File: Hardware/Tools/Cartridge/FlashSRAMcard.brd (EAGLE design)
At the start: 47.9 x 47.9 mm, 18 parts, among them IC1 AS29CF160B-55TIN, IC2 74LS595D, IC3 74LS244DW, IC5 74AHC1G04DBV, IC6 74AHC1G32DBV, IC7 74AHC1G32DBV

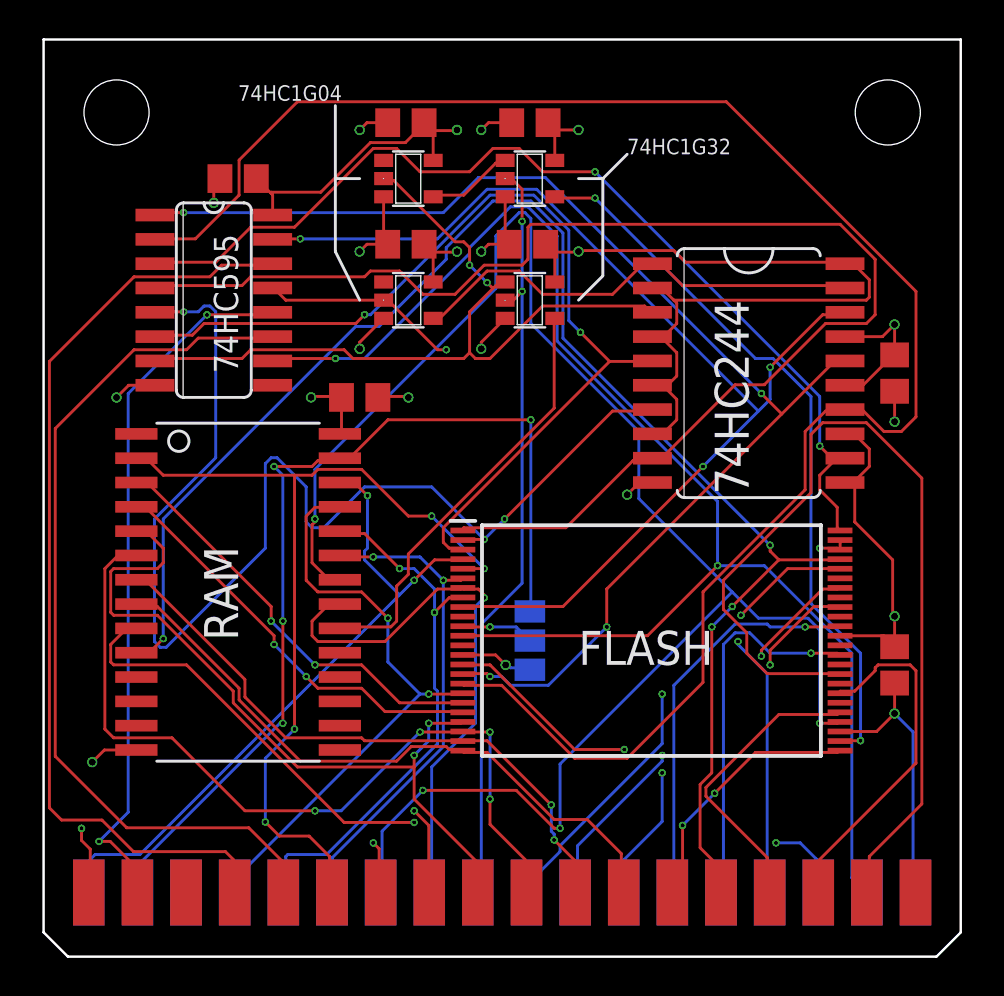
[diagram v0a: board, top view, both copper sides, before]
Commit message: more sram cart changes
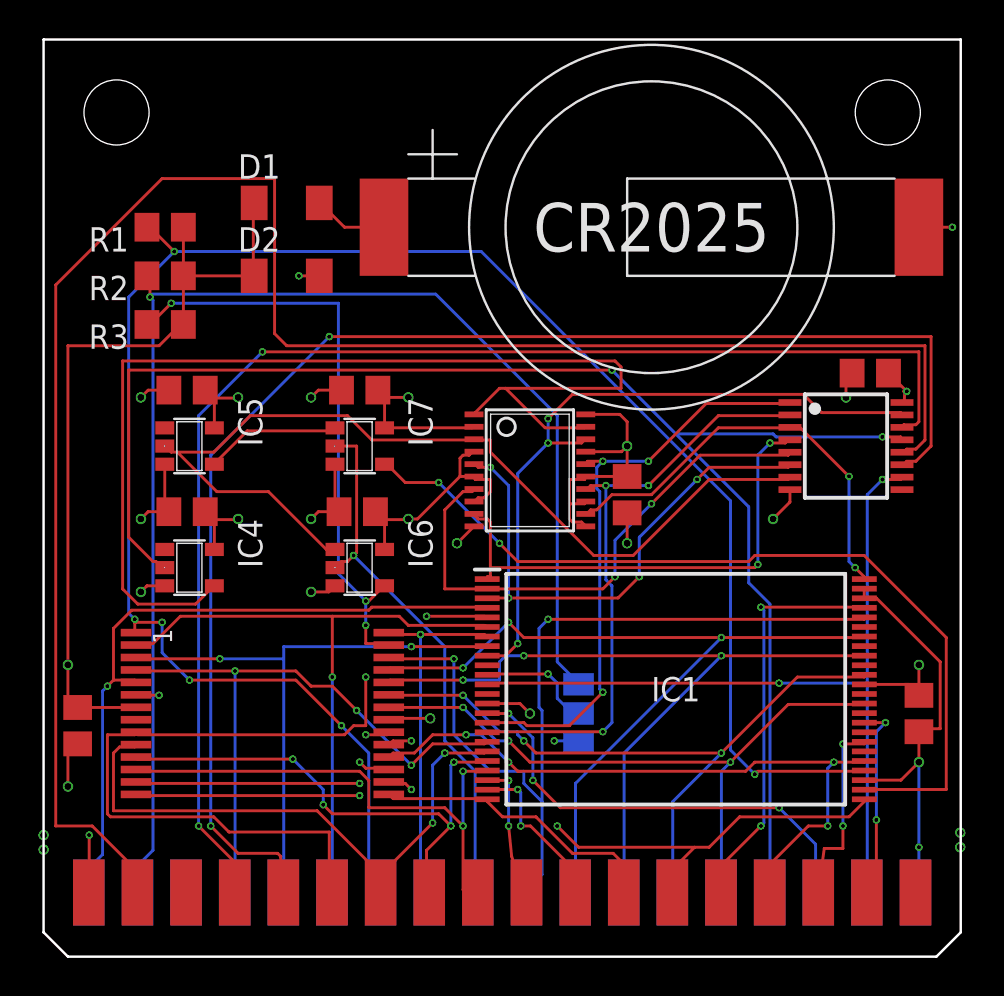
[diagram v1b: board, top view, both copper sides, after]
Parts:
- removed VCC: 74AHC1G04DBV, 74xx-little-us:SOT23-5
- added D1, D2: (no value), semicon-smd-ipc:MELF-MLL34
- added IC4: 74AHC1G04DBV, 74xx-little-us:SOT23-5
- added R1, R2, R3: (no value), rcl:R0805
- added U$3: BATTERY2025-SMD, 0_gametankparts:CR2025-SMD
- IC2: value 74LS595D -> 74HC595; device 74xx-us:SO16 -> 0_gametankparts:TSSOP16
- IC3: value 74LS244DW -> 74HC244; device 74xx-us:SO20W -> 0_gametankparts:TSSOP20
- U$2: value SRAM_32KSOP28 -> SRAM_32KTSOP28; device 0_gametankparts:SO28-3 -> 0_gametankparts:TSOP10X14
- moved C3 34.5 mm to (43.2, 30.5)
- moved IC2 33.9 mm to (41.9, 26.7)
- moved C4 22.6 mm to (1.78, 12.1), turned to 270 degrees
- moved IC5 18.1 mm to (7.62, 26.7)
- moved C5 18.1 mm to (7.49, 29.6)
- moved C7 18.1 mm to (7.49, 23.2)
- moved C8 16.6 mm to (16.4, 23.2)
- moved C6 16.6 mm to (16.5, 29.6)
- moved IC6 16.6 mm to (16.5, 20.3)
- moved IC7 16.6 mm to (16.5, 26.7)
- moved C2 15.3 mm to (30.5, 24.1)
- moved IC3 12.5 mm to (25.4, 25.4)
- moved U$2 6.48 mm to (11.4, 12.7)
- moved W 4.58 mm to (27.9, 12.7)
- moved IC1 2.84 mm to (33.0, 14.0)
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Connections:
- new net N$5: D1.2, U$3.P$1
- new net N$6: C4.1, D1.1, D2.1, R1.1, R2.1, R3.1, U$2.7
- net !BANKING: now also IC4.2; no longer VCC.2
- net !OE: now also R1.2, U$2.1; no longer U$2.22
- net !WE: now also R2.2, U$2.6; no longer U$2.27
- net A-1: now also U$2.17; no longer U$2.10
- net A0: now also U$2.16; no longer U$2.9
- net A1: now also U$2.15; no longer U$2.8
- net A10: now also U$2.2; no longer U$2.23
- net A11: now also U$2.9; no longer U$2.2
- net A12: now also U$2.5; no longer U$2.26
- net A2: now also U$2.14; no longer U$2.7
- net A3: now also U$2.13; no longer U$2.6
- net A4: now also U$2.12; no longer U$2.5
- net A5: now also U$2.11; no longer U$2.4
- net A6: now also U$2.10; no longer U$2.3
- net A7: now also U$2.4; no longer U$2.25
- net A8: now also U$2.3; no longer U$2.24
- net A9: now also U$2.28; no longer U$2.21
- net D0: now also U$2.18
- net D1: now also U$2.19
- net D2: now also U$2.20
- net D3: now also U$2.22
- net D4: now also U$2.23
- net D5: now also U$2.24
- net D6: now also U$2.25
- net D7: now also U$2.26
- net GND: now also IC4.3, U$2.21, U$3.P$2; no longer U$2.14, VCC.3
- net N$1: now also IC4.4; no longer VCC.4
- net N$2: now also R3.2, U$2.27; no longer U$2.20
- net VCC: now also D2.2, IC4.5; no longer C4.1, U$2.28, VCC.5
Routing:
- net A17: track 92.6 -> 31.5 mm, vias 0 -> 3
- net BANK_DONE: track 37.2 -> 97.1 mm, vias 2 -> 0
- net GND: track 43.2 -> 97.1 mm, vias 14 -> 17
- net A15: track 70.9 -> 25.9 mm, vias 0 -> 2
- net N$6: track 0.00 -> 41.3 mm, vias 0 -> 1
- net A18: track 67.1 -> 31.2 mm, vias 4 -> 3
- net A14: track 63.3 -> 28.2 mm, vias 3 -> 2
- net N$1: track 24.2 -> 58.0 mm
- net !BANKING: track 45.8 -> 79.2 mm
- net !RESET: track 76.3 -> 42.9 mm
- net A-1: track 81.3 -> 48.3 mm, vias 4 -> 3
- net A16: track 52.8 -> 22.4 mm
- net BANK_CLK: track 46.3 -> 73.4 mm, vias 0 -> 2
- net A19: track 58.6 -> 35.8 mm
- net !WE: track 50.2 -> 72.8 mm, vias 4 -> 2
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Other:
- board text removed: "74HC1G04"
- board text removed: "74HC1G32"
- board text removed: "74HC244"
- board text removed: "74HC595"
- board text removed: "FLASH"
- board text removed: "RAM"
